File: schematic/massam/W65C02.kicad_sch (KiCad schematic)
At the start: 25 parts, among them U100B W65C02SxPL, U101B SST39SF512, U102B UT62256PC-70LL, U103B GAL20L8, U104B 74AHC04, Y100B 14.310Mhz

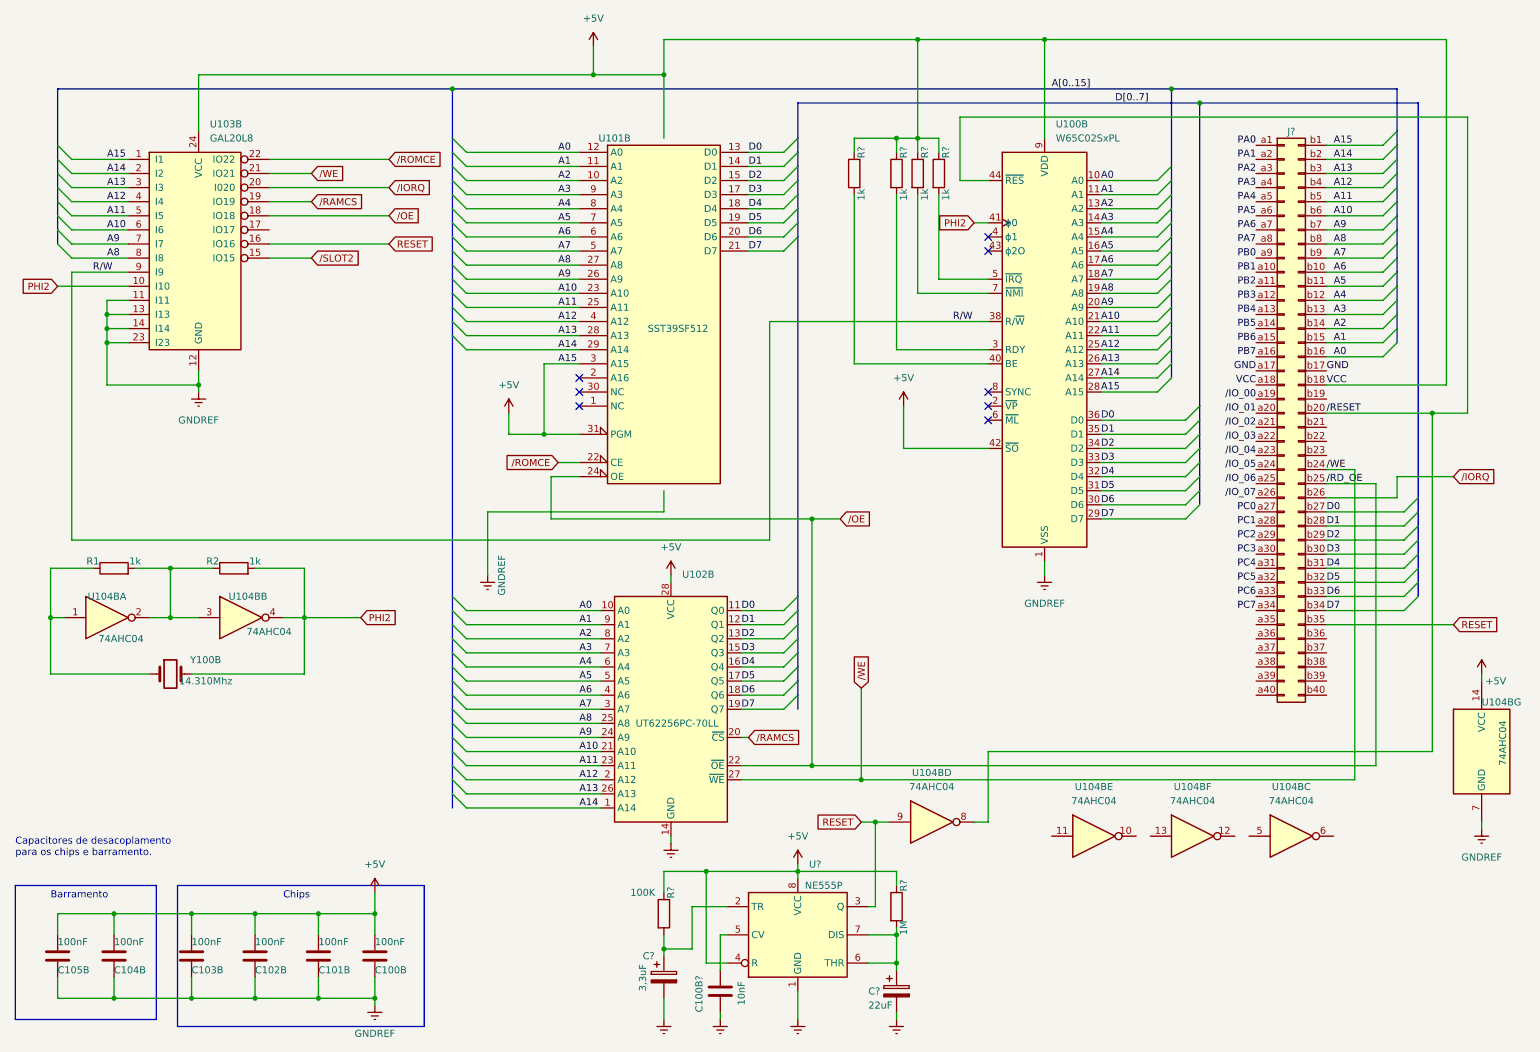
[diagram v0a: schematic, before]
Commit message: Alinhamento com biosmon
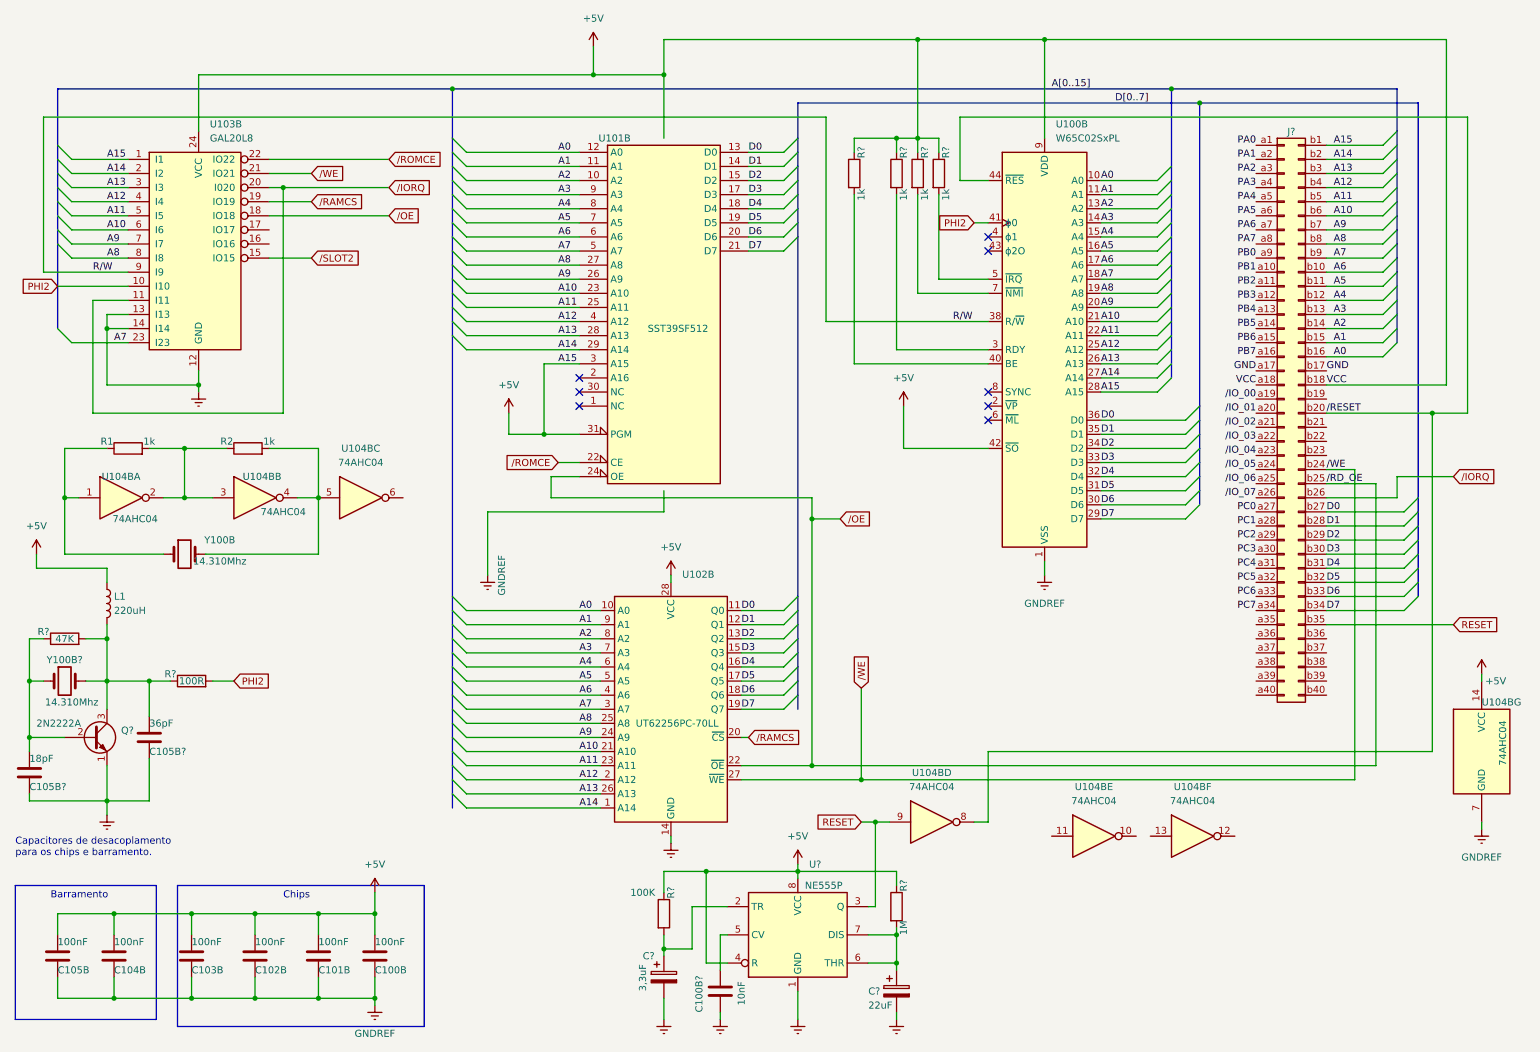
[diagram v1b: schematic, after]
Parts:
- added C105B?: 18pF, symbol Device:C
- added C105B?: 36pF, symbol Device:C
- added L1: 220uH, symbol Device:L
- added Q?: 2N2222A, Package_TO_SOT_THT:TO-39-3, symbol Transistor_BJT:2N2219
- added R?: 100R, symbol Device:R
- added R?: 47K, symbol Device:R
- added Y100B?: 14.310Mhz, symbol Device:Crystal
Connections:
- net +5V: now also L1.1
- net A7: now also U103B.23 (I23)
- net GND: now also C105B?.2, C105B?.2, Q?.1 (E); no longer U103B.11 (I11), U103B.23 (I23)
- net PHI2: now also R?.2; no longer R2.2, U104B.4, Y100B.2
- net RESET: no longer U103B.16 (IO16)
- net /IORQ: now also U103B.11 (I11)
- net at U104B.5: now also R2.2, U104B.4, Y100B.2
- new net: C105B?.1, L1.2, Q?.3 (C), R?.1, R?.2, Y100B?.2
- new net: C105B?.1, Q?.2 (B), R?.1, Y100B?.1
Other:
- moved on the sheet: R1, R2, U104BA, U104BB, U104BC, Y100B
